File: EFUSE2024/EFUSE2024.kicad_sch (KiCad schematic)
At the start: 4 parts, among them U1 TPS26631PWP, U2 TPS26631PWP, U3 TPS26631PWP, U4 TPS26631PWP

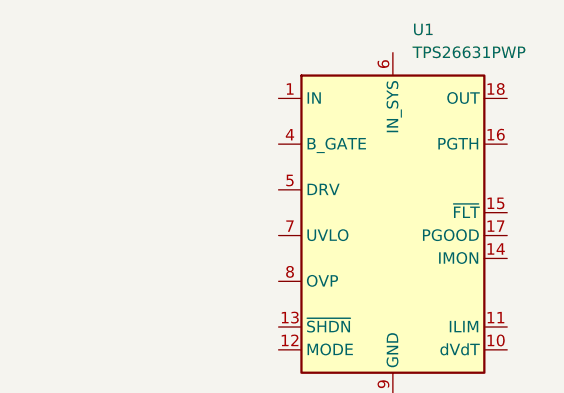
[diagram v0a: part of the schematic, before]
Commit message: Update EFUSE2024.kicad_sch
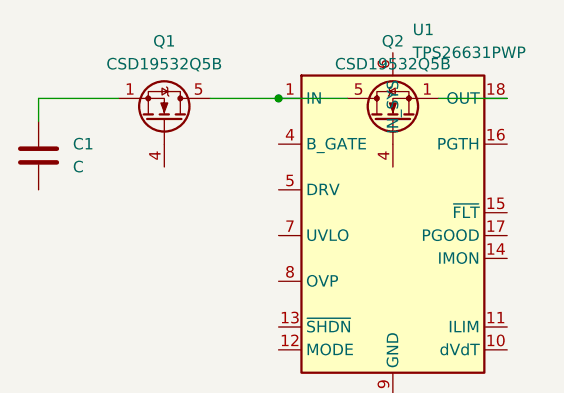
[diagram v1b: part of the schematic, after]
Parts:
- added C1: C, symbol Device:C
- added Q1, Q2: CSD19532Q5B, Package_TO_SOT_SMD:TDSON-8-1, symbol Transistor_FET:CSD19532Q5B
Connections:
- net at U1.1 (IN), U1.2 (IN), U1.3 (IN): now also Q1.5 (D), Q2.5 (D)
- net at U1.18 (OUT), U1.19 (OUT), U1.20 (OUT): now also Q2.1 (S), Q2.2 (S), Q2.3 (S)
- new net: C1.1, Q1.1 (S), Q1.2 (S), Q1.3 (S)

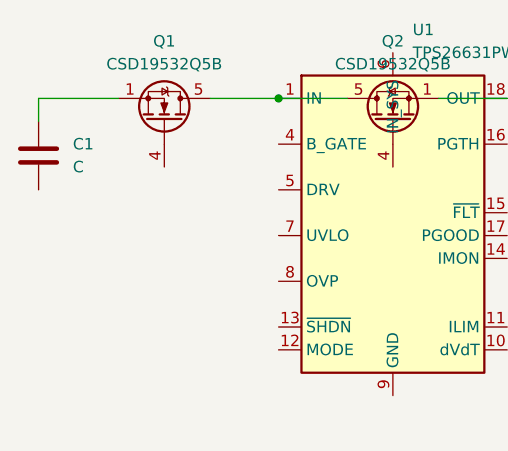
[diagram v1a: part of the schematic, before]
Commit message: Update EFUSE2024.kicad_sch
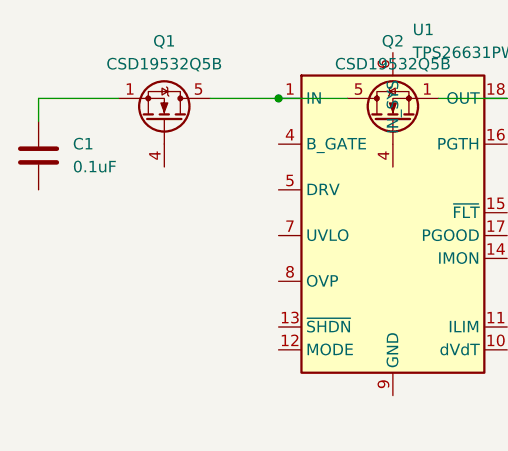
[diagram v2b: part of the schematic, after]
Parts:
- C1: value C -> 0.1uF
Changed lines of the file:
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@@
 			)
 		)
-		(property "Value" "C"
+		(property "Value" "0.1uF"
 			(at 110.49 27.9399 0)
 			(effects

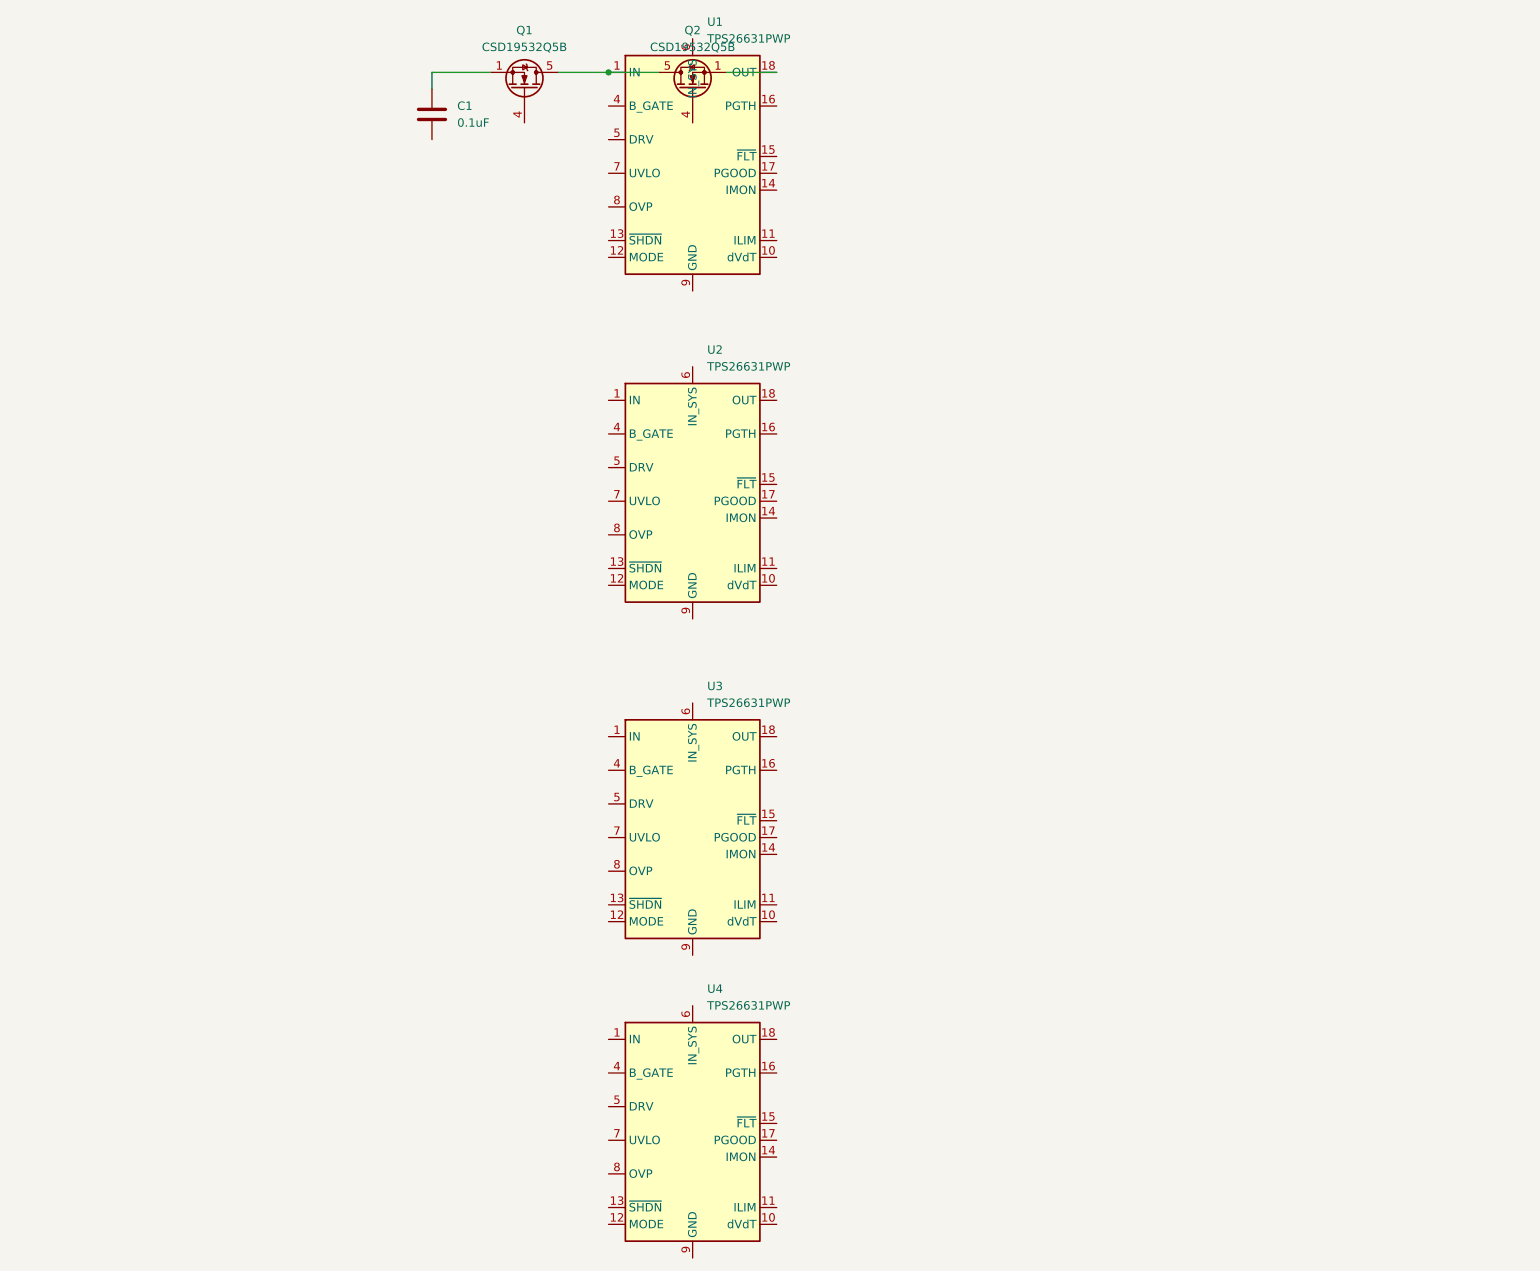
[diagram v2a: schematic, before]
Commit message: test
something
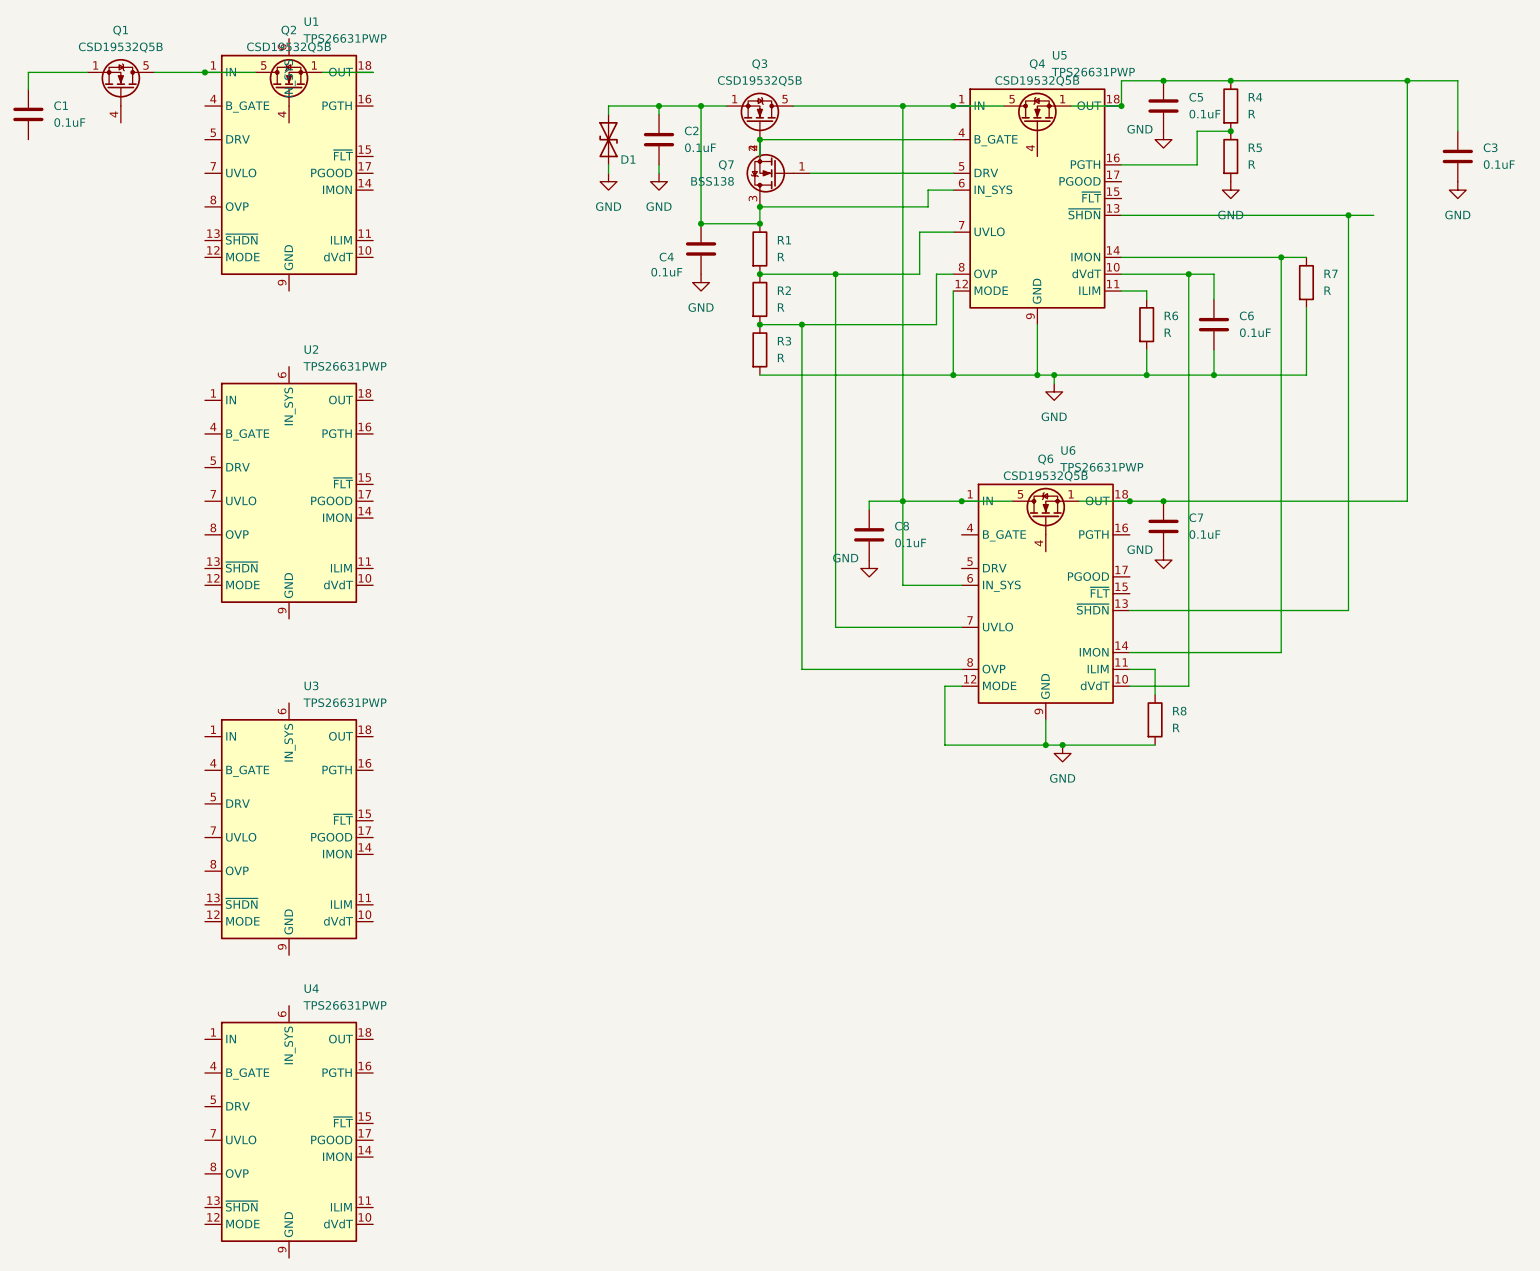
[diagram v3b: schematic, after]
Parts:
- added C2, C3, C4, C5, C6, C7, C8: 0.1uF, symbol Device:C
- added D1: 1.5SMCxxCA, Diode_SMD:D_SMC, symbol Diode:1.5SMCxxCA
- added Q3, Q4, Q6: CSD19532Q5B, Package_TO_SOT_SMD:TDSON-8-1, symbol Transistor_FET:CSD19532Q5B
- added Q7: BSS138, Package_TO_SOT_SMD:SOT-23, symbol Transistor_FET:BSS138
- added R1, R2, R3, R4, R5, R6, R7, R8: R, symbol Device:R
- added U5, U6: TPS26631PWP, Package_SO:HTSSOP-20-1EP_4.4x6.5mm_P0.65mm_EP3.4x6.5mm_Mask2.96x2.96mm_ThermalVias, symbol Power_Management:TPS26631PWP
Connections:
- new net: R2.2, R3.1, U5.8 (OVP), U6.8 (OVP)
- new net: C2.1, C4.1, D1.2 (A2), Q3.1 (S), Q3.2 (S), Q3.3 (S), Q7.3 (D), R1.1, U5.6 (IN_SYS)
- new net: R6.1, U5.11 (ILIM)
- new net: C8.1, Q3.5 (D), Q4.5 (D), Q6.5 (D), U5.1 (IN), U5.2 (IN), U5.3 (IN), U6.1 (IN), U6.2 (IN), U6.3 (IN), U6.6 (IN_SYS)
- new net: C3.1, C5.1, C7.1, Q4.1 (S), Q4.2 (S), Q4.3 (S), Q6.1 (S), Q6.2 (S), Q6.3 (S), R4.1, U5.18 (OUT), U5.19 (OUT), U5.20 (OUT), U6.18 (OUT), U6.19 (OUT), U6.20 (OUT)
- new net: R4.2, R5.1, U5.16 (PGTH)
- new net: C6.1, U5.10 (dVdT), U6.10 (dVdT)
- new net: R8.1, U6.11 (ILIM)
- new net: U5.13 (~{SHDN}), U6.13 (~{SHDN})
- new net: R7.1, U5.14 (IMON), U6.14 (IMON)
- new net: R1.2, R2.1, U5.7 (UVLO), U6.7 (UVLO)
- new net: Q3.4 (G), Q7.2 (S), U5.4 (B_GATE)
- new net: Q7.1 (G), U5.5 (DRV)
- new net GND: C2.2, C3.2, C4.2, C5.2, C6.2, C7.2, C8.2, D1.1 (A1), R3.2, R5.2, R6.2, R7.2, R8.2, U5.12 (MODE), U5.21 (GND), U5.9 (GND), U6.12 (MODE), U6.21 (GND), U6.9 (GND)
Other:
- moved on the sheet: C1, Q1, Q2, U1, U2, U3, U4

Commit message: For Nitya
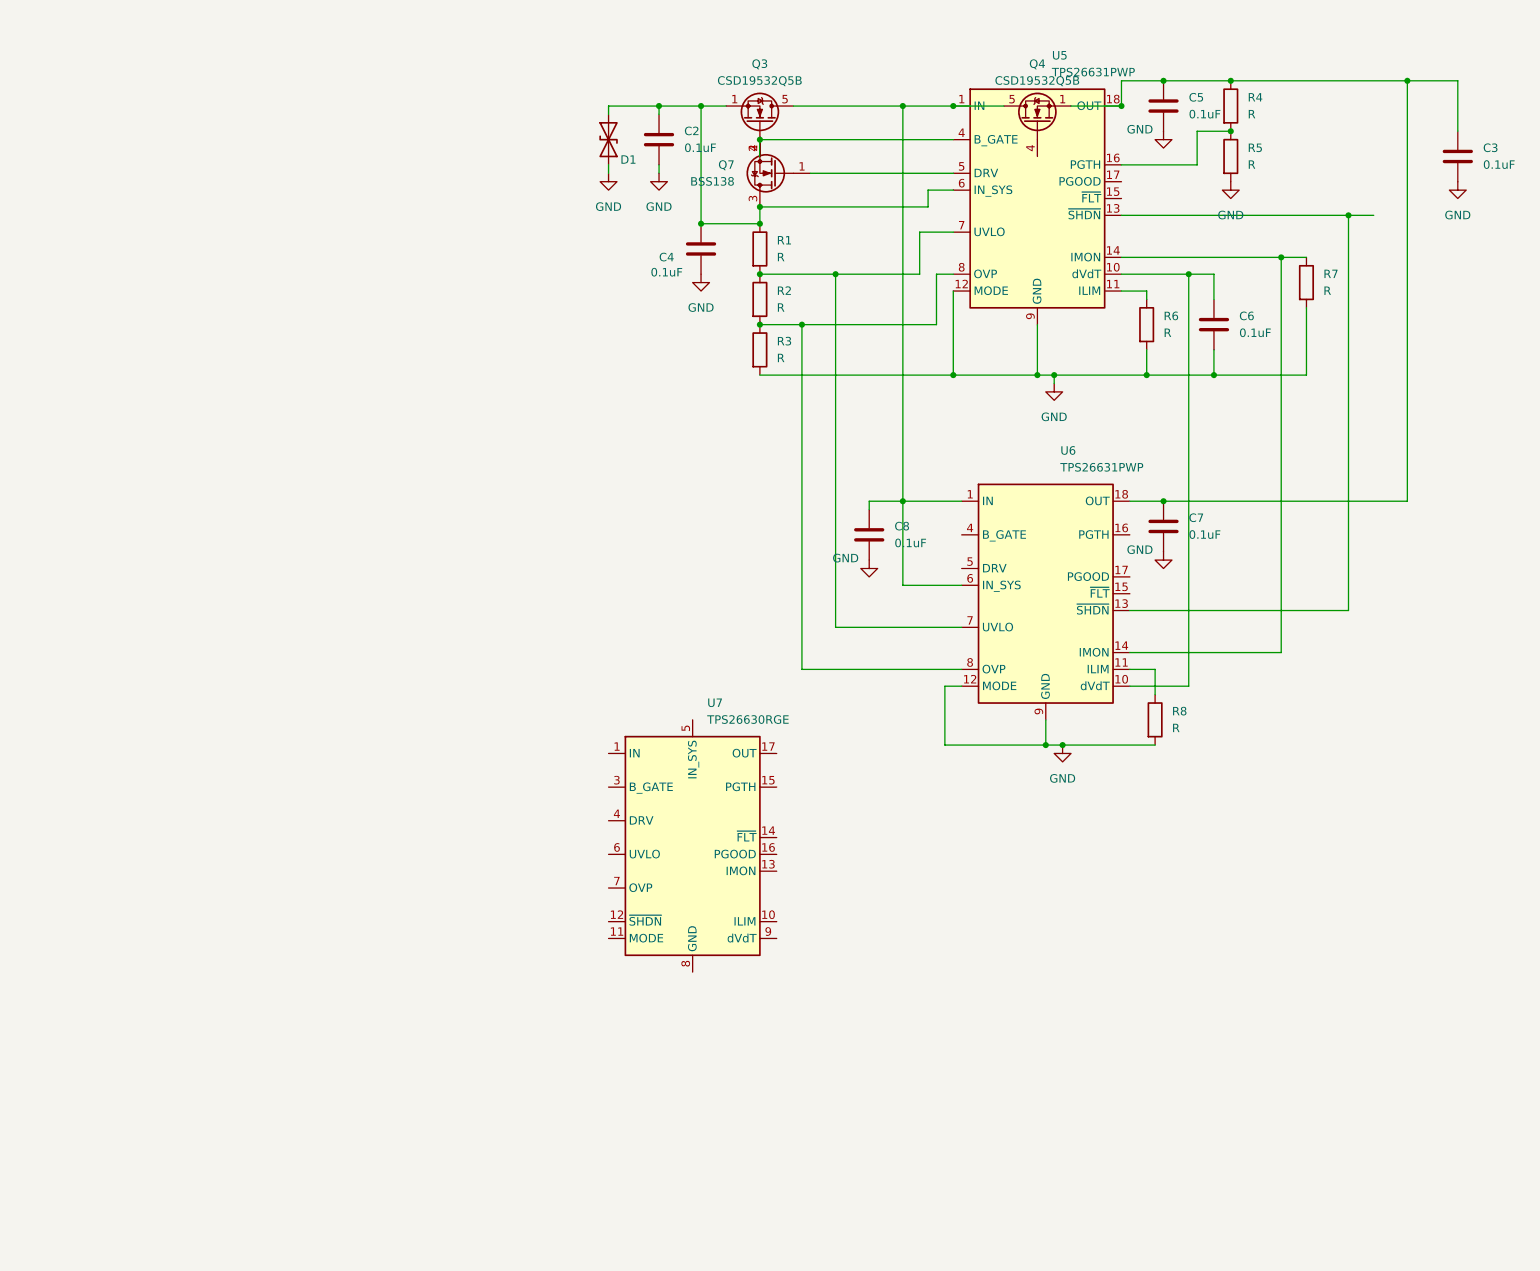
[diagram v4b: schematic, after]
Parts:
- removed C1: 0.1uF, symbol Device:C
- removed Q1, Q2, Q6: CSD19532Q5B, Package_TO_SOT_SMD:TDSON-8-1, symbol Transistor_FET:CSD19532Q5B
- removed U1, U2, U3, U4: TPS26631PWP, Package_SO:HTSSOP-20-1EP_4.4x6.5mm_P0.65mm_EP3.4x6.5mm_Mask2.96x2.96mm_ThermalVias, symbol Power_Management:TPS26631PWP
- added U7: TPS26630RGE, Package_DFN_QFN:Texas_RGE0024H_VQFN-24-1EP_4x4mm_P0.5mm_EP2.7x2.7mm_ThermalVias, symbol Power_Management:TPS26630RGE
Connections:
- new net: U7.1 (IN), U7.2 (IN)
- new net: U7.17 (OUT), U7.18 (OUT)
- new net: U7.25 (GND), U7.8 (GND)
